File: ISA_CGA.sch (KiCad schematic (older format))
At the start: 29 parts, among them U1 74S112, U11 74LS74, U12 74LS393, U13 74LS08, U14 74LS32, U15 74LS00, U16 74LS04, U2 74LS74, U20 74LS04, U22 74LS51, U23 74LS32, U25 74LS00, U26 74LS04, U27 74LS51, U28 74LS10, U29 74S04, U3 74S86, U30 74LS32, U31 74S08, U41 74LS08, U42 74LS86, U46 74LS00, U47 74LS51, U48 74LS51, U49 74LS02, U6 74LS04, U62 74LS125, U65 74LS02, U68 74LS86

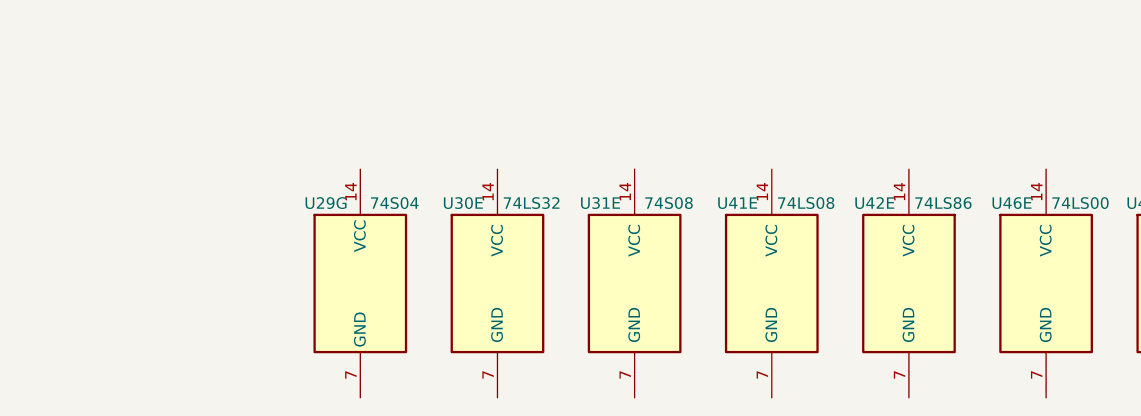
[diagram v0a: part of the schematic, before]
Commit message: More sheet 5
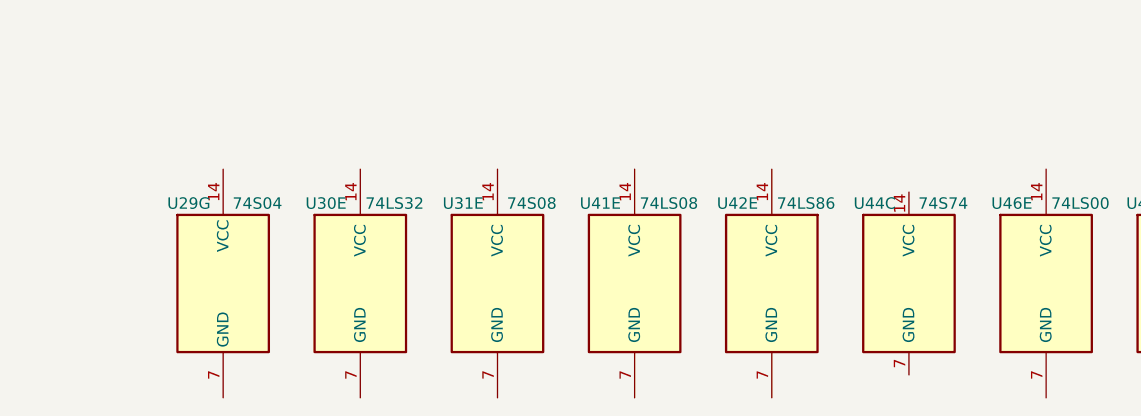
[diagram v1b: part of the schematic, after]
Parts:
- added U44: 74S74, Package_DIP:DIP-14_W7.62mm_LongPads, symbol 74xx:74LS74
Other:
- moved on the sheet: U29G, U30E, U31E, U41E, U42E
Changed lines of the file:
@@
 L 74xx:74LS08 U?
 U 5 1 61D13A76
-P 4150 5150
+P 3550 5150
 AR Path="/60463C10/61D13A76" Ref="U?"  Part="3"
 AR Path="/61D13A76" Ref="U31"  Part="5"
-F 0 "U31" H 4000 5500 50  0000 C CNN
-F 1 "74S08" H 4300 5500 50  0000 C CNN
-F 2 "Package_DIP:DIP-14_W7.62mm_LongPads" H 4150 5150 50  0001 C CNN
-F 3 "http://www.ti.com/lit/gpn/sn74LS08" H 4150 5150 50  0001 C CNN
-	5    4150 5150
+F 0 "U31" H 3400 5500 50  0000 C CNN
+F 1 "74S08" H 3700 5500 50  0000 C CNN
+F 2 "Package_DIP:DIP-14_W7.62mm_LongPads" H 3550 5150 50  0001 C CNN
+F 3 "http://www.ti.com/lit/gpn/sn74LS08" H 3550 5150 50  0001 C CNN
+	5    3550 5150
 	1    0    0    -1
 $EndComp
@@
 L 74xx:74LS86 U?
 U 5 1 629C2DFD
-P 5350 5150
+P 4750 5150
 AR Path="/60463C10/629C2DFD" Ref="U?"  Part="4"
 AR Path="/60463C57/629C2DFD" Ref="U?"  Part="1"
 AR Path="/629C2DFD" Ref="U42"  Part="5"
-F 0 "U42" H 5500 5500 50  0000 C CNN
-F 1 "74LS86" H 5200 5500 50  0000 C CNN
-F 2 "Package_DIP:DIP-14_W7.62mm_LongPads" H 5350 5150 50  0001 C CNN
-F 3 "74xx/74ls86.pdf" H 5350 5150 50  0001 C CNN
-	5    5350 5150
+F 0 "U42" H 4900 5500 50  0000 C CNN
+F 1 "74LS86" H 4600 5500 50  0000 C CNN
+F 2 "Package_DIP:DIP-14_W7.62mm_LongPads" H 4750 5150 50  0001 C CNN
+F 3 "74xx/74ls86.pdf" H 4750 5150 50  0001 C CNN
+	5    4750 5150
 	-1   0    0    -1
 $EndComp
@@
 L 74xx:74LS32 U?
 U 5 1 62AC6F3C
-P 3550 5150
+P 2950 5150
 AR Path="/60463C57/62AC6F3C" Ref="U?"  Part="3"
 AR Path="/62AC6F3C" Ref="U30"  Part="5"
-F 0 "U30" H 3400 5500 50  0000 C CNN
-F 1 "74LS32" H 3700 5500 50  0000 C CNN
-F 2 "" H 3550 5150 50  0001 C CNN
-F 3 "http://www.ti.com/lit/gpn/sn74LS32" H 3550 5150 50  0001 C CNN
-	5    3550 5150
+F 0 "U30" H 2800 5500 50  0000 C CNN
+F 1 "74LS32" H 3100 5500 50  0000 C CNN
+F 2 "" H 2950 5150 50  0001 C CNN
+F 3 "http://www.ti.com/lit/gpn/sn74LS32" H 2950 5150 50  0001 C CNN
+	5    2950 5150
 	1    0    0    -1
 $EndComp
@@
 L 74xx:74LS08 U?
 U 5 1 62CA5B30
-P 4750 5150
+P 4150 5150
 AR Path="/60463C57/62CA5B30" Ref="U?"  Part="4"
 AR Path="/62CA5B30" Ref="U41"  Part="5"
-F 0 "U41" H 4600 5500 50  0000 C CNN
-F 1 "74LS08" H 4900 5500 50  0000 C CNN
-F 2 "Package_DIP:DIP-14_W7.62mm_LongPads" H 4750 5150 50  0001 C CNN
-F 3 "http://www.ti.com/lit/gpn/sn74LS08" H 4750 5150 50  0001 C CNN
-	5    4750 5150
+F 0 "U41" H 4000 5500 50  0000 C CNN
+F 1 "74LS08" H 4300 5500 50  0000 C CNN
+F 2 "Package_DIP:DIP-14_W7.62mm_LongPads" H 4150 5150 50  0001 C CNN
+F 3 "http://www.ti.com/lit/gpn/sn74LS08" H 4150 5150 50  0001 C CNN
+	5    4150 5150
 	1    0    0    -1
 $EndComp
@@
 L 74xx:74LS04 U?
 U 7 1 63CE58E6
-P 2950 5150
+P 2350 5150
 AR Path="/60463C57/63CE58E6" Ref="U?"  Part="6"
 AR Path="/60463CC5/63CE58E6" Ref="U?"  Part="4"
 AR Path="/63CE58E6" Ref="U29"  Part="7"
-F 0 "U29" H 2800 5500 50  0000 C CNN
-F 1 "74S04" H 3100 5500 50  0000 C CNN
-F 2 "Package_DIP:DIP-14_W7.62mm_LongPads" H 2950 5150 50  0001 C CNN
-F 3 "http://www.ti.com/lit/gpn/sn74LS04" H 2950 5150 50  0001 C CNN
-	7    2950 5150
+F 0 "U29" H 2200 5500 50  0000 C CNN
+F 1 "74S04" H 2500 5500 50  0000 C CNN
+F 2 "Package_DIP:DIP-14_W7.62mm_LongPads" H 2350 5150 50  0001 C CNN
+F 3 "http://www.ti.com/lit/gpn/sn74LS04" H 2350 5150 50  0001 C CNN
+	7    2350 5150
 	1    0    0    -1
 $EndComp
@@
 	1    0    0    -1
 $EndComp
+$Comp
+L 74xx:74LS74 U?
+U 3 1 64BD6305
+P 5350 5150
+AR Path="/60463CF3/64BD6305" Ref="U?"  Part="1"
+AR Path="/64BD6305" Ref="U44"  Part="3"
+F 0 "U44" H 5200 5500 50  0000 C CNN
+F 1 "74S74" H 5500 5500 50  0000 C CNN
+F 2 "Package_DIP:DIP-14_W7.62mm_LongPads" H 5350 5150 50  0001 C CNN
+F 3 "74xx/74hc_hct74.pdf" H 5350 5150 50  0001 C CNN
+	3    5350 5150
+	1    0    0    -1
+$EndComp
